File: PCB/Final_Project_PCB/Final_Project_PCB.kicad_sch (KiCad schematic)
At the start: 34 parts

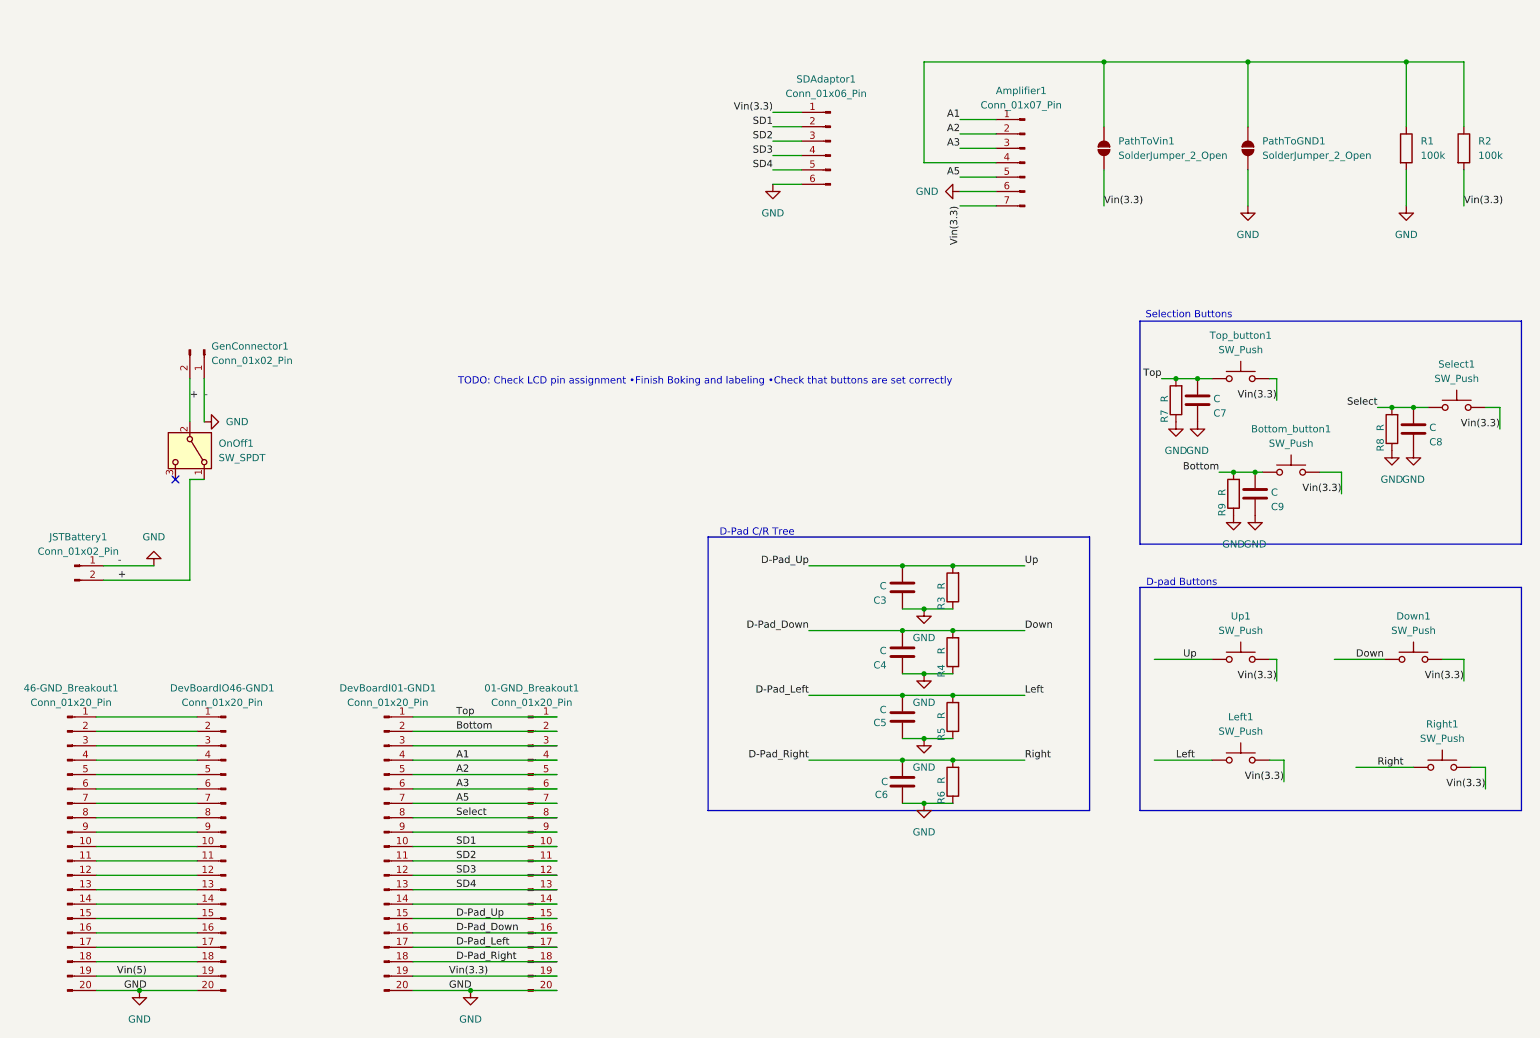
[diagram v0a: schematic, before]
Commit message: Current KiCAD November 4 5PM
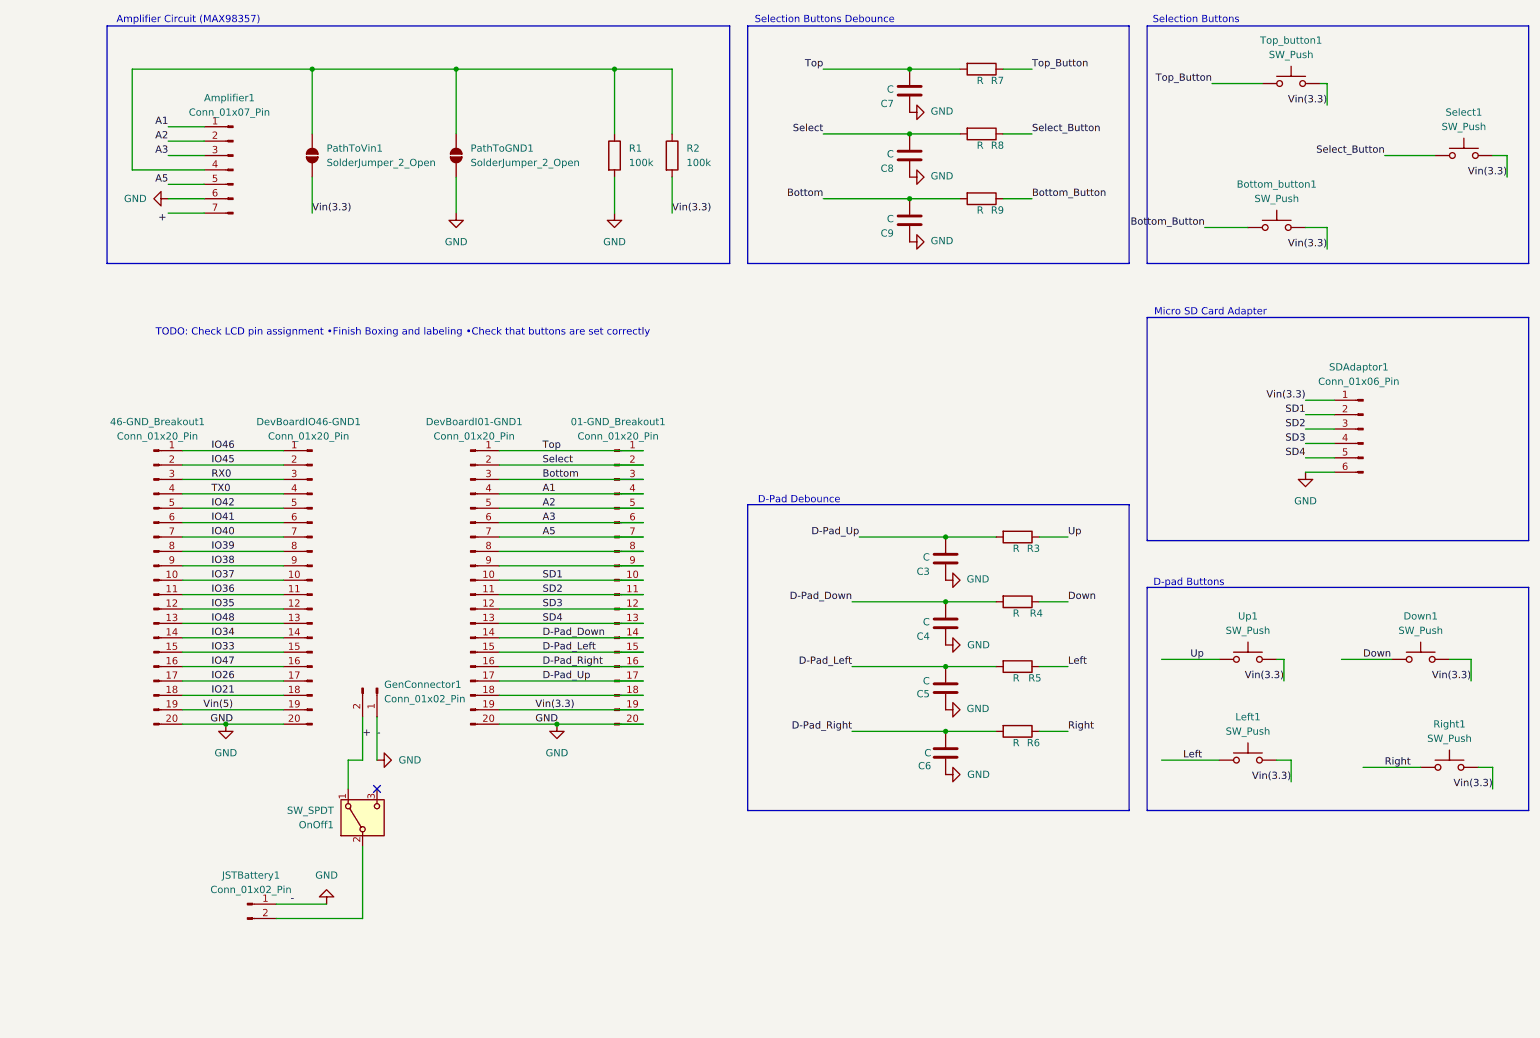
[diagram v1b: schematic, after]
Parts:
- C3, C4, C5, C6, C7, C8, C9: footprint Capacitor_SMD:C_0805_2012Metric -> Capacitor_SMD:C_0805_2012Metric_Pad1.18x1.45mm_HandSolder
- R1, R2, R3, R4, R5, R6, R7, R8, R9: footprint Resistor_SMD:R_0201_0603Metric -> Resistor_SMD:R_0805_2012Metric_Pad1.20x1.40mm_HandSolder
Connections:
- net +: now also Amplifier1.7 (Pin_7); no longer JSTBattery1.2 (Pin_2), OnOff1.2 (B)
- net Bottom: now also 01-GND_Breakout1.3 (Pin_3), DevBoardI01-GND1.3 (Pin_3); no longer 01-GND_Breakout1.2 (Pin_2), Bottom_button1.1, DevBoardI01-GND1.2 (Pin_2)
- net D-Pad_Down: now also 01-GND_Breakout1.14 (Pin_14), DevBoardI01-GND1.14 (Pin_14); no longer 01-GND_Breakout1.16 (Pin_16), DevBoardI01-GND1.16 (Pin_16), Down1.1
- net D-Pad_Left: now also 01-GND_Breakout1.15 (Pin_15), DevBoardI01-GND1.15 (Pin_15); no longer 01-GND_Breakout1.17 (Pin_17), DevBoardI01-GND1.17 (Pin_17), Left1.1
- net D-Pad_Right: now also 01-GND_Breakout1.16 (Pin_16), DevBoardI01-GND1.16 (Pin_16); no longer 01-GND_Breakout1.18 (Pin_18), DevBoardI01-GND1.18 (Pin_18), Right1.1
- net D-Pad_Up: now also 01-GND_Breakout1.17 (Pin_17), DevBoardI01-GND1.17 (Pin_17); no longer 01-GND_Breakout1.15 (Pin_15), DevBoardI01-GND1.15 (Pin_15), Up1.1
- net GND: no longer R3.1, R4.1, R5.1, R6.1, R7.1, R8.1, R9.1
- net Select: now also 01-GND_Breakout1.2 (Pin_2), DevBoardI01-GND1.2 (Pin_2); no longer 01-GND_Breakout1.8 (Pin_8), DevBoardI01-GND1.8 (Pin_8), Select1.1
- net Top: no longer Top_button1.1
- net Vin(3.3): no longer Amplifier1.7 (Pin_7)
- net IO46: now reaches 46-GND_Breakout1.1 (Pin_1), DevBoardIO46-GND1.1 (Pin_1)
- net IO37: now reaches 46-GND_Breakout1.10 (Pin_10), DevBoardIO46-GND1.10 (Pin_10)
- net IO36: now reaches 46-GND_Breakout1.11 (Pin_11), DevBoardIO46-GND1.11 (Pin_11)
- net IO35: now reaches 46-GND_Breakout1.12 (Pin_12), DevBoardIO46-GND1.12 (Pin_12)
- net IO48: now reaches 46-GND_Breakout1.13 (Pin_13), DevBoardIO46-GND1.13 (Pin_13)
- net IO34: now reaches 46-GND_Breakout1.14 (Pin_14), DevBoardIO46-GND1.14 (Pin_14)
- net IO33: now reaches 46-GND_Breakout1.15 (Pin_15), DevBoardIO46-GND1.15 (Pin_15)
- net IO47: now reaches 46-GND_Breakout1.16 (Pin_16), DevBoardIO46-GND1.16 (Pin_16)
- net IO26: now reaches 46-GND_Breakout1.17 (Pin_17), DevBoardIO46-GND1.17 (Pin_17)
- net IO21: now reaches 46-GND_Breakout1.18 (Pin_18), DevBoardIO46-GND1.18 (Pin_18)
- net IO45: now reaches 46-GND_Breakout1.2 (Pin_2), DevBoardIO46-GND1.2 (Pin_2)
- net RX0: now reaches 46-GND_Breakout1.3 (Pin_3), DevBoardIO46-GND1.3 (Pin_3)
- net TX0: now reaches 46-GND_Breakout1.4 (Pin_4), DevBoardIO46-GND1.4 (Pin_4)
- net IO42: now reaches 46-GND_Breakout1.5 (Pin_5), DevBoardIO46-GND1.5 (Pin_5)
- net IO41: now reaches 46-GND_Breakout1.6 (Pin_6), DevBoardIO46-GND1.6 (Pin_6)
- net IO40: now reaches 46-GND_Breakout1.7 (Pin_7), DevBoardIO46-GND1.7 (Pin_7)
- net IO39: now reaches 46-GND_Breakout1.8 (Pin_8), DevBoardIO46-GND1.8 (Pin_8)
- net IO38: now reaches 46-GND_Breakout1.9 (Pin_9), DevBoardIO46-GND1.9 (Pin_9)
- new net: 01-GND_Breakout1.18 (Pin_18), DevBoardI01-GND1.18 (Pin_18)
- new net: 01-GND_Breakout1.8 (Pin_8), DevBoardI01-GND1.8 (Pin_8)
- new net: JSTBattery1.2 (Pin_2), OnOff1.2 (B)
- new net Bottom_Button: Bottom_button1.1, R9.1
- new net Down: Down1.1, R4.1
- new net Left: Left1.1, R5.1
- new net Right: R6.1, Right1.1
- new net Select_Button: R8.1, Select1.1
- new net Top_Button: R7.1, Top_button1.1
- new net Up: R3.1, Up1.1
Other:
- note added: "Amplifier Circuit (MAX98357)"
- note added: "D-Pad Debounce"
- note added: "Micro SD Card Adapter"
- note added: "Selection Buttons Debounce"
- note added: "TODO: Check LCD pin assignment •Finish Boxing and labeling •Check that buttons are set correctly"
- note removed: "D-Pad C/R Tree"
- note removed: "TODO: Check LCD pin assignment •Finish Boking and labeling •Check that buttons are set correctly"
- moved on the sheet: 01-GND_Breakout1, 46-GND_Breakout1, Amplifier1, Bottom_button1, C3, C4, C5, C6, DevBoardI01-GND1, DevBoardIO46-GND1, Down1, GenConnector1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
